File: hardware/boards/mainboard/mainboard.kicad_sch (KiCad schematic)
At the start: 4 parts, among them J1 Conn_01x03, U1 RP2040

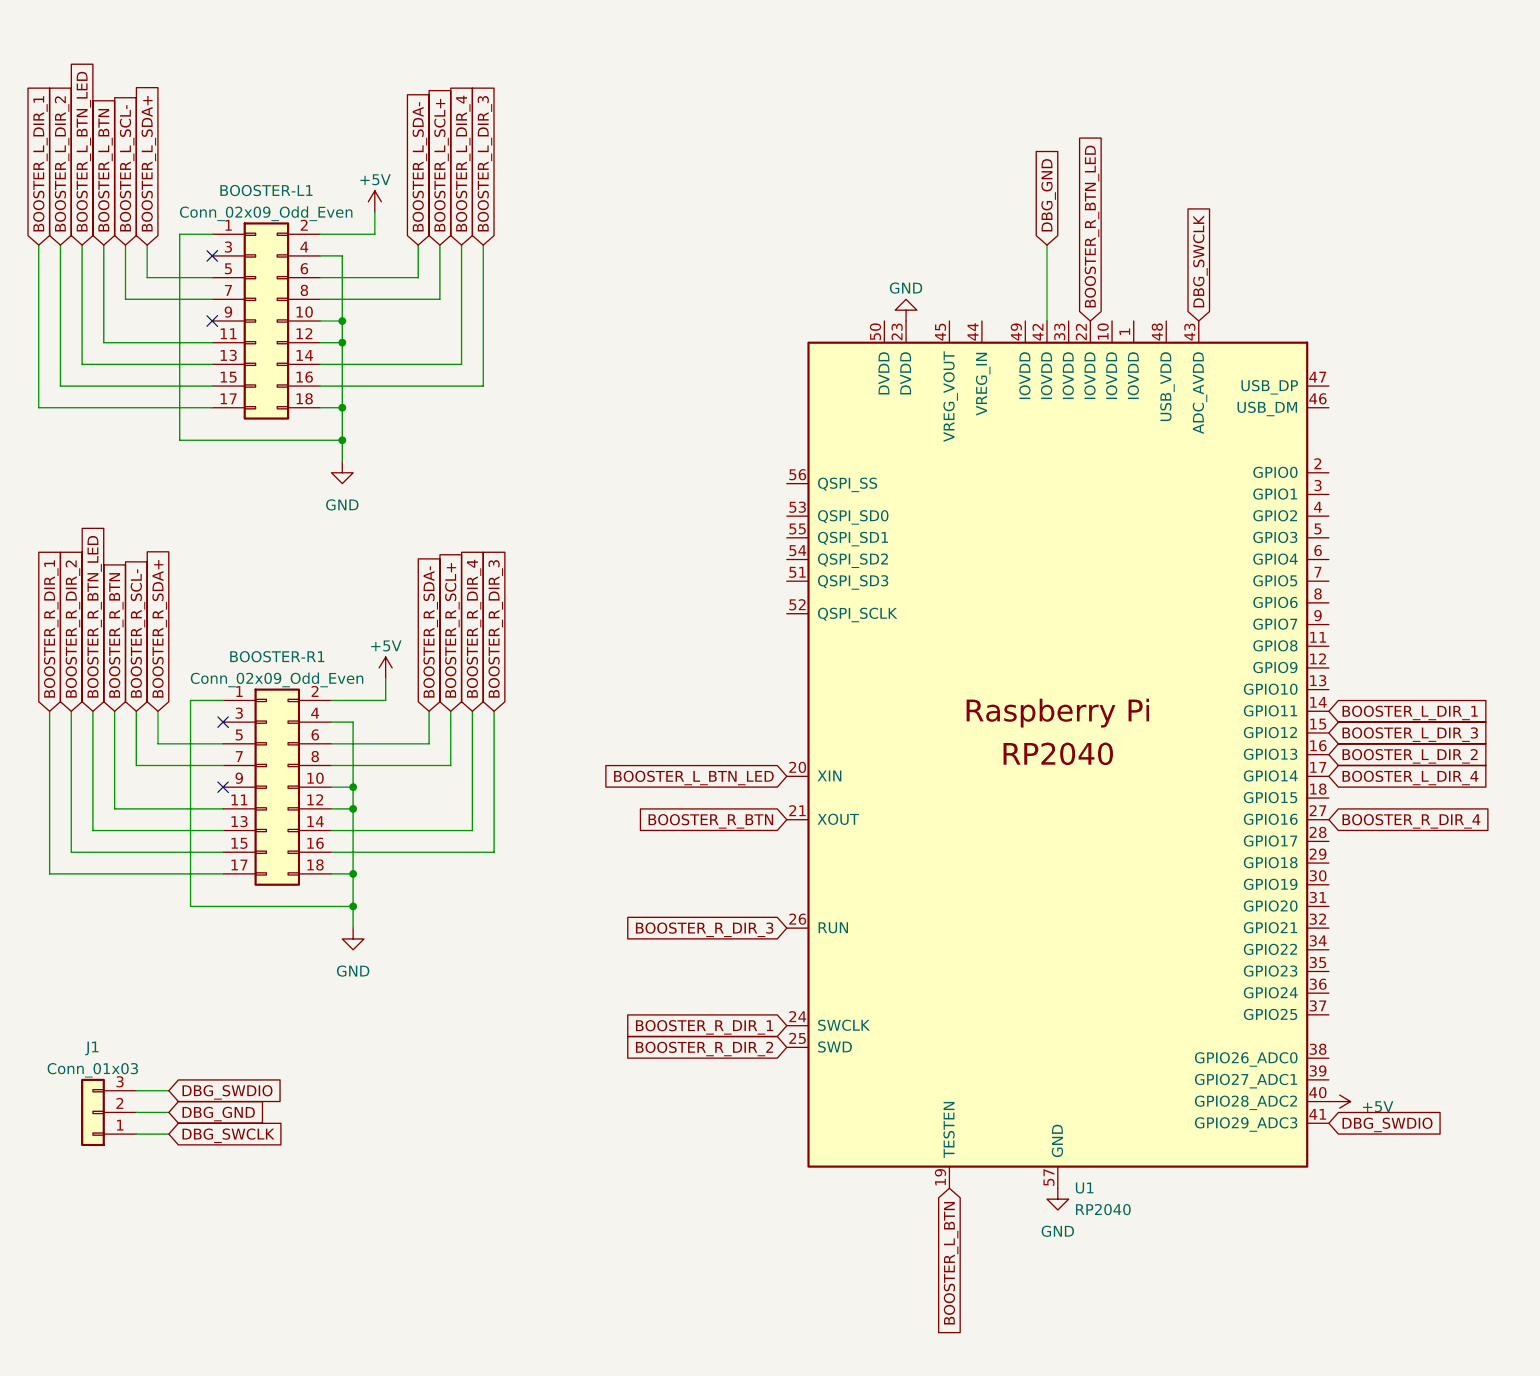
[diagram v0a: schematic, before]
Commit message: refactor(hardware): refactor mainboard
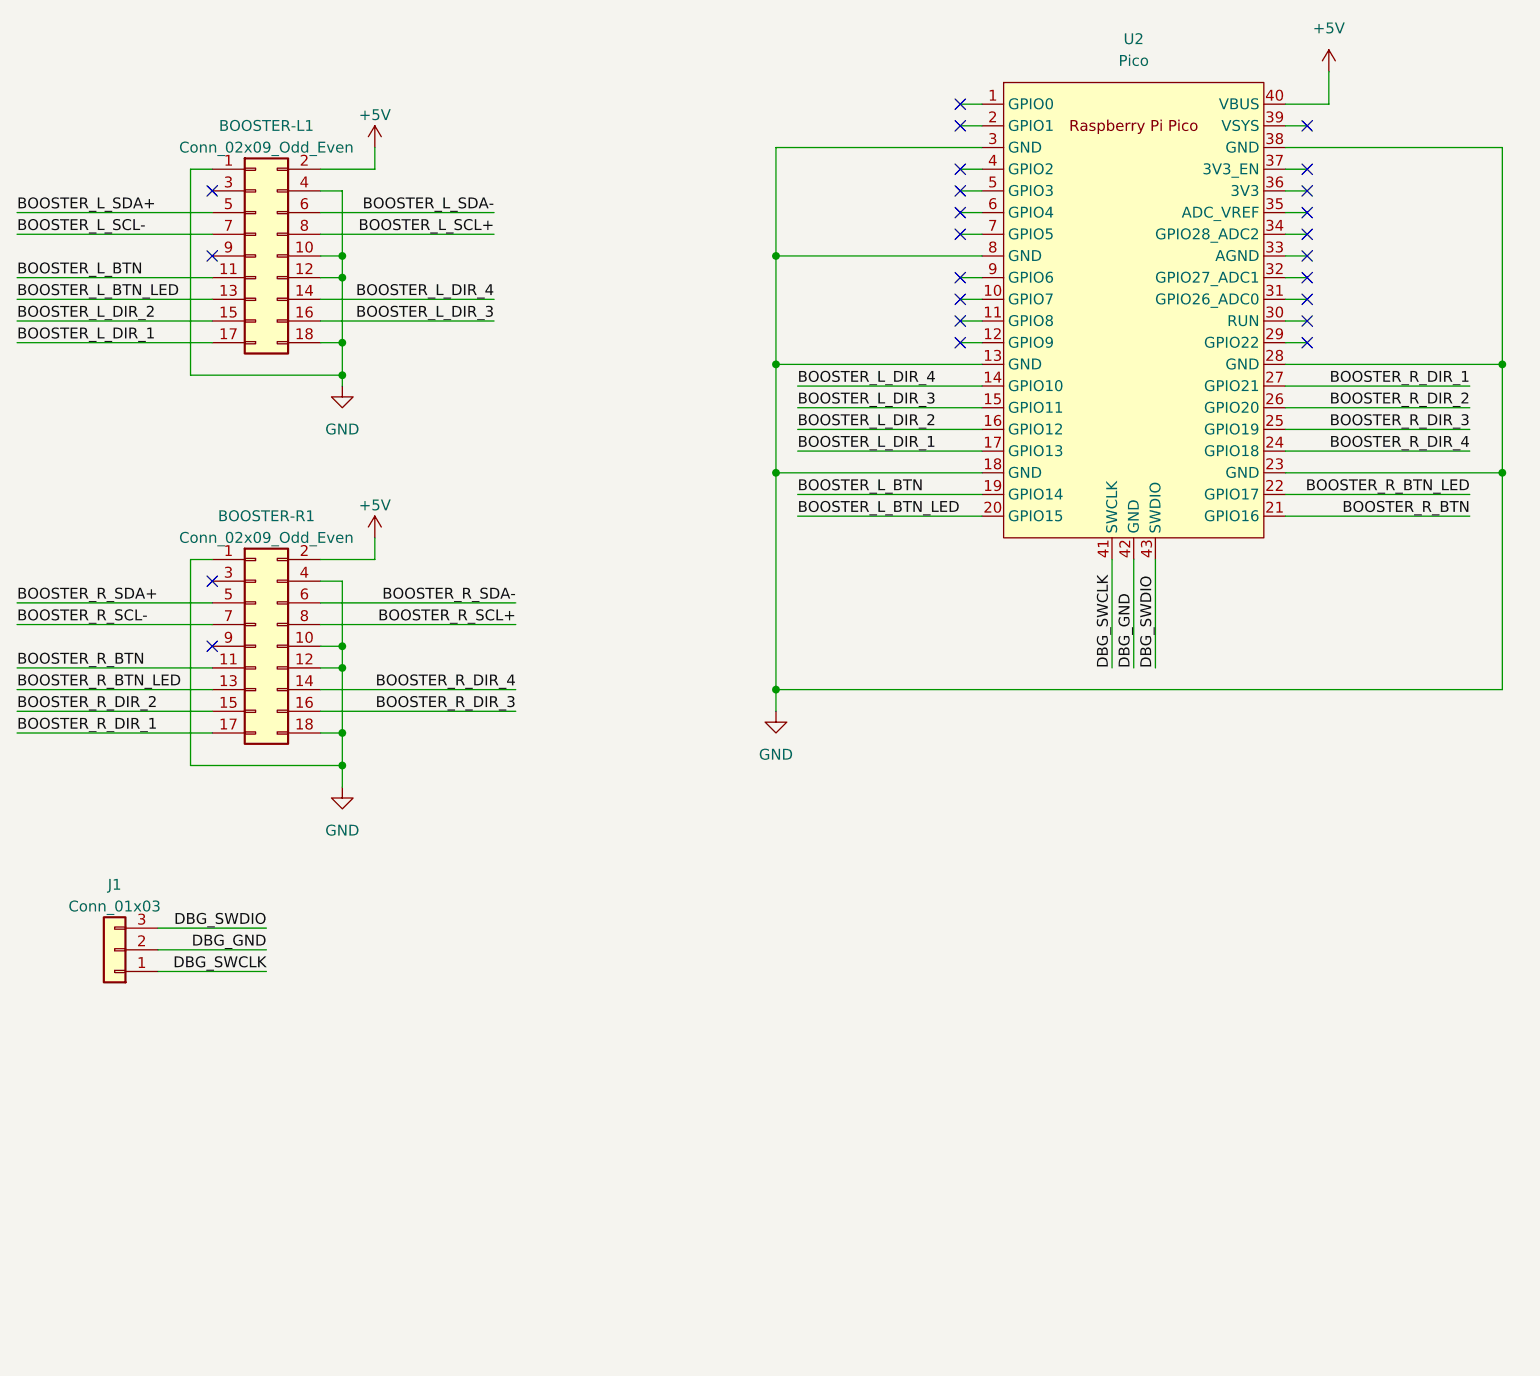
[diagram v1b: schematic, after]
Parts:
- removed U1: RP2040, MCU_RaspberryPi_and_Boards:RPi_Pico_SMD_TH, symbol MCU_RaspberryPi_and_Boards:RP2040
- added U2: Pico, MCU_RaspberryPi_and_Boards:RPi_Pico_SMD_TH_Clean, symbol MCU_RaspberryPi_and_Boards:Pico
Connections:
- net +5V: now also U2.40 (VBUS)
- net BOOSTER_L_BTN: now also U2.19 (GPIO14)
- net BOOSTER_L_BTN_LED: now also U2.20 (GPIO15)
- net BOOSTER_L_DIR_1: now also U2.17 (GPIO13)
- net BOOSTER_L_DIR_2: now also U2.16 (GPIO12)
- net BOOSTER_L_DIR_3: now also U2.15 (GPIO11)
- net BOOSTER_L_DIR_4: now also U2.14 (GPIO10)
- net BOOSTER_R_BTN: now also U2.21 (GPIO16)
- net BOOSTER_R_BTN_LED: now also U2.22 (GPIO17)
- net BOOSTER_R_DIR_1: now also U2.27 (GPIO21)
- net BOOSTER_R_DIR_2: now also U2.26 (GPIO20)
- net BOOSTER_R_DIR_3: now also U2.25 (GPIO19)
- net BOOSTER_R_DIR_4: now also U2.24 (GPIO18)
- net DBG_GND: now also U2.42 (GND)
- net DBG_SWCLK: now also U2.41 (SWCLK)
- net DBG_SWDIO: now also U2.43 (SWDIO)
- net GND: now also U2.13 (GND), U2.18 (GND), U2.23 (GND), U2.28 (GND), U2.3 (GND), U2.38 (GND), U2.8 (GND)
- no-connect marks 4 -> 24
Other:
- title: Booster Brain -> Mainboard
- moved on the sheet: BOOSTER-L1, BOOSTER-R1, J1
